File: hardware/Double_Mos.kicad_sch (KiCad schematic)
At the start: 12 parts, among them U14 AOZ5276QI, U15 AOZ5276QI

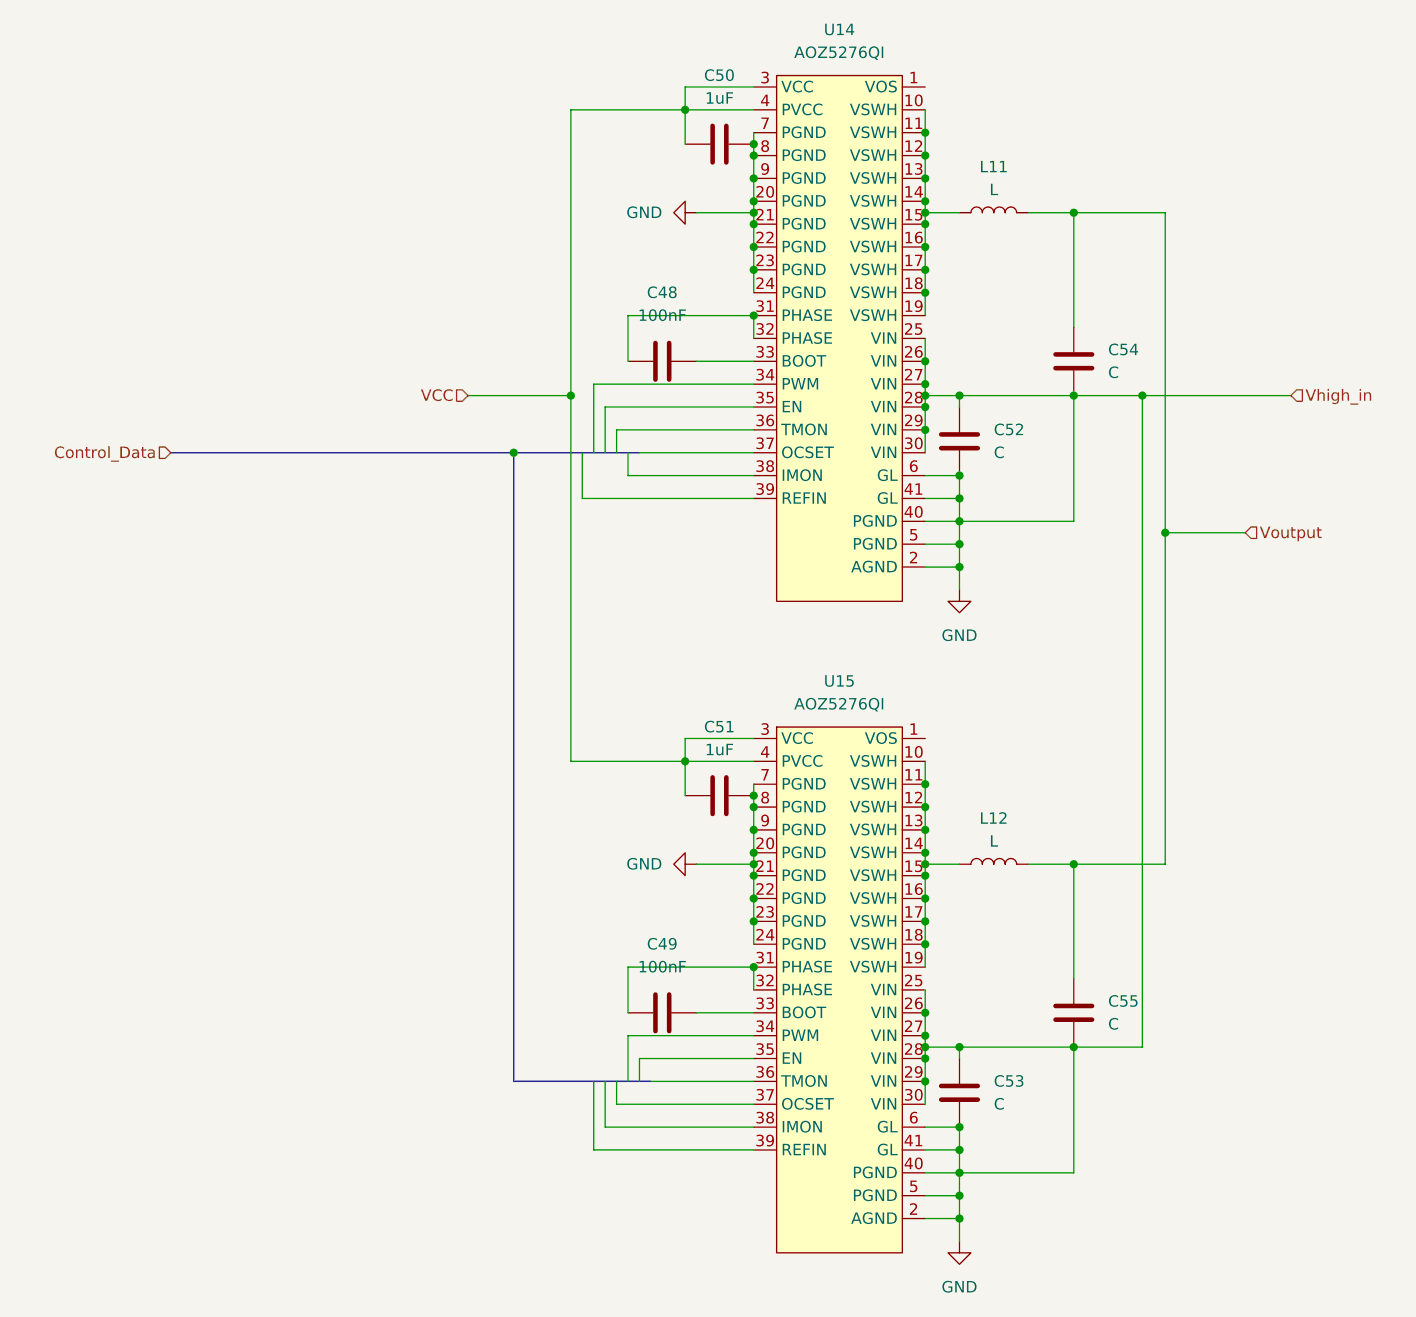
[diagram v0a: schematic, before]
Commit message: Revert "chore(schematic): Update references"
This reverts commit 2cda2d22061e90f93ddb38c43ecf32892cd7b43c.
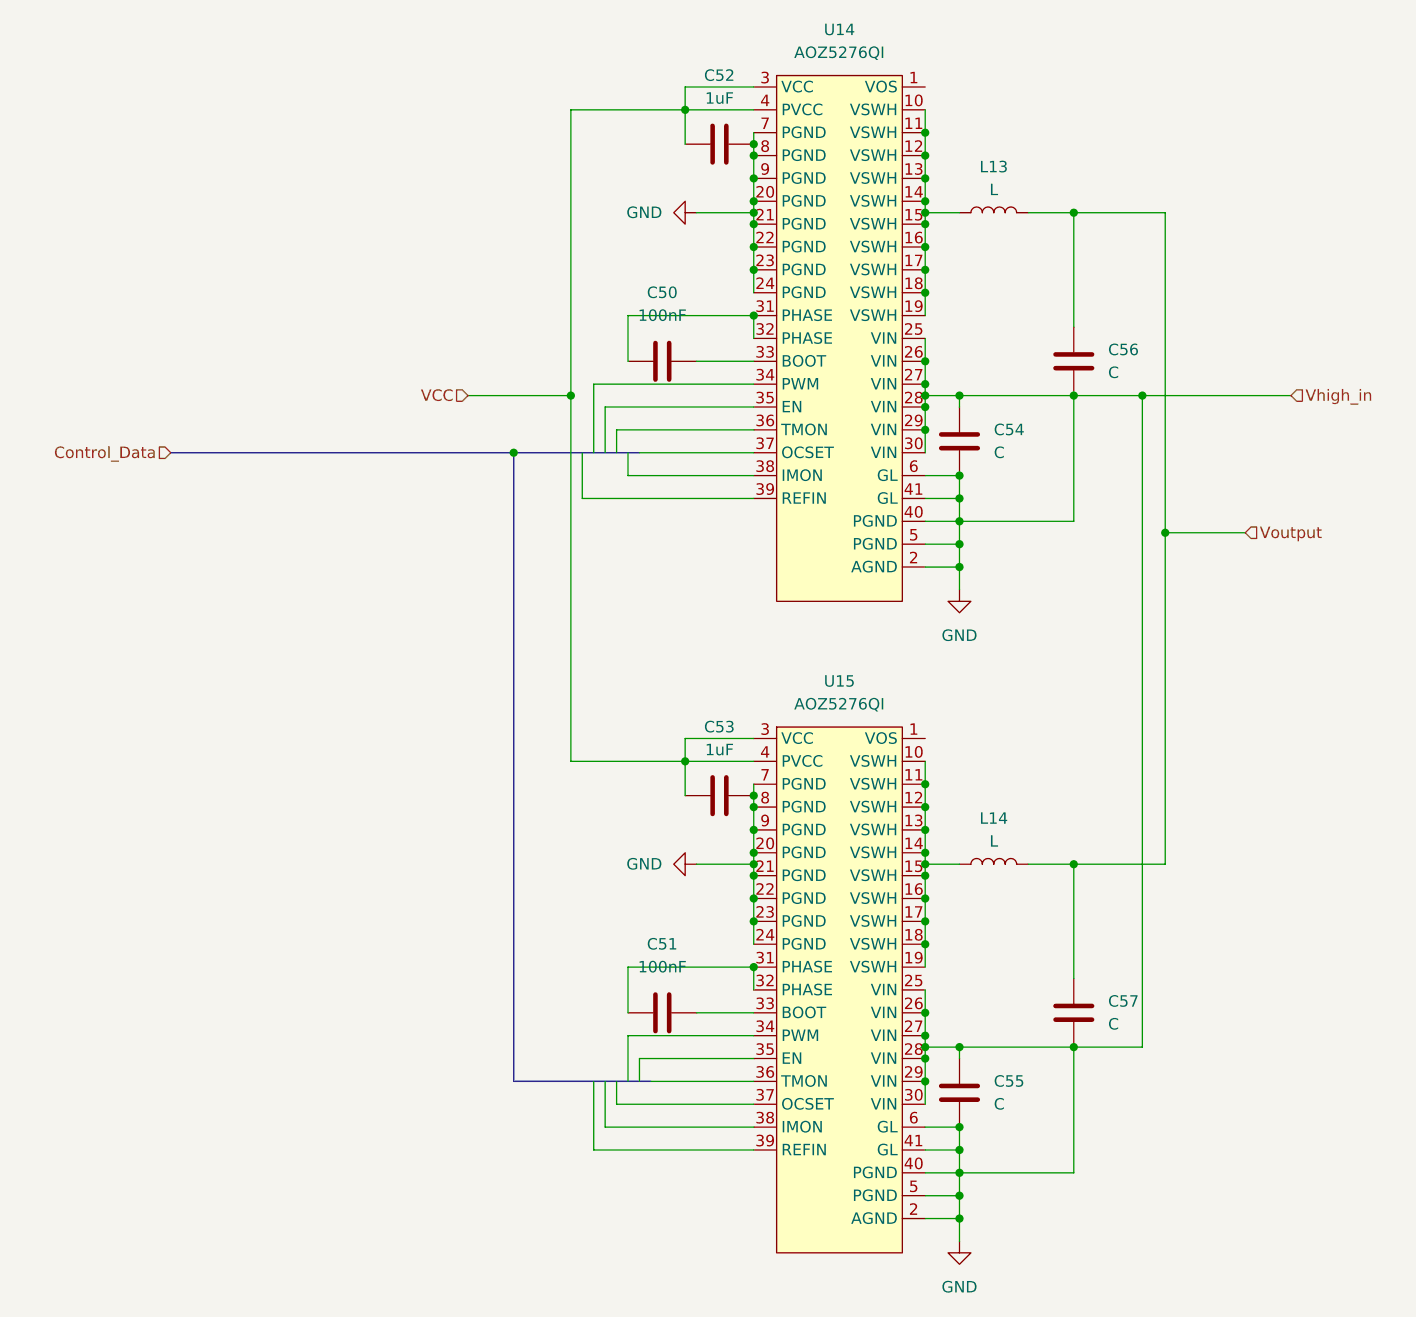
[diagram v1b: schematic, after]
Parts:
- renumbered C48 to C50, C49 to C51, C50 to C52, C51 to C53, C52 to C54, C53 to C55, C54 to C56, C55 to C57, L11 to L13, L12 to L14

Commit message: chore(schematic): Update references
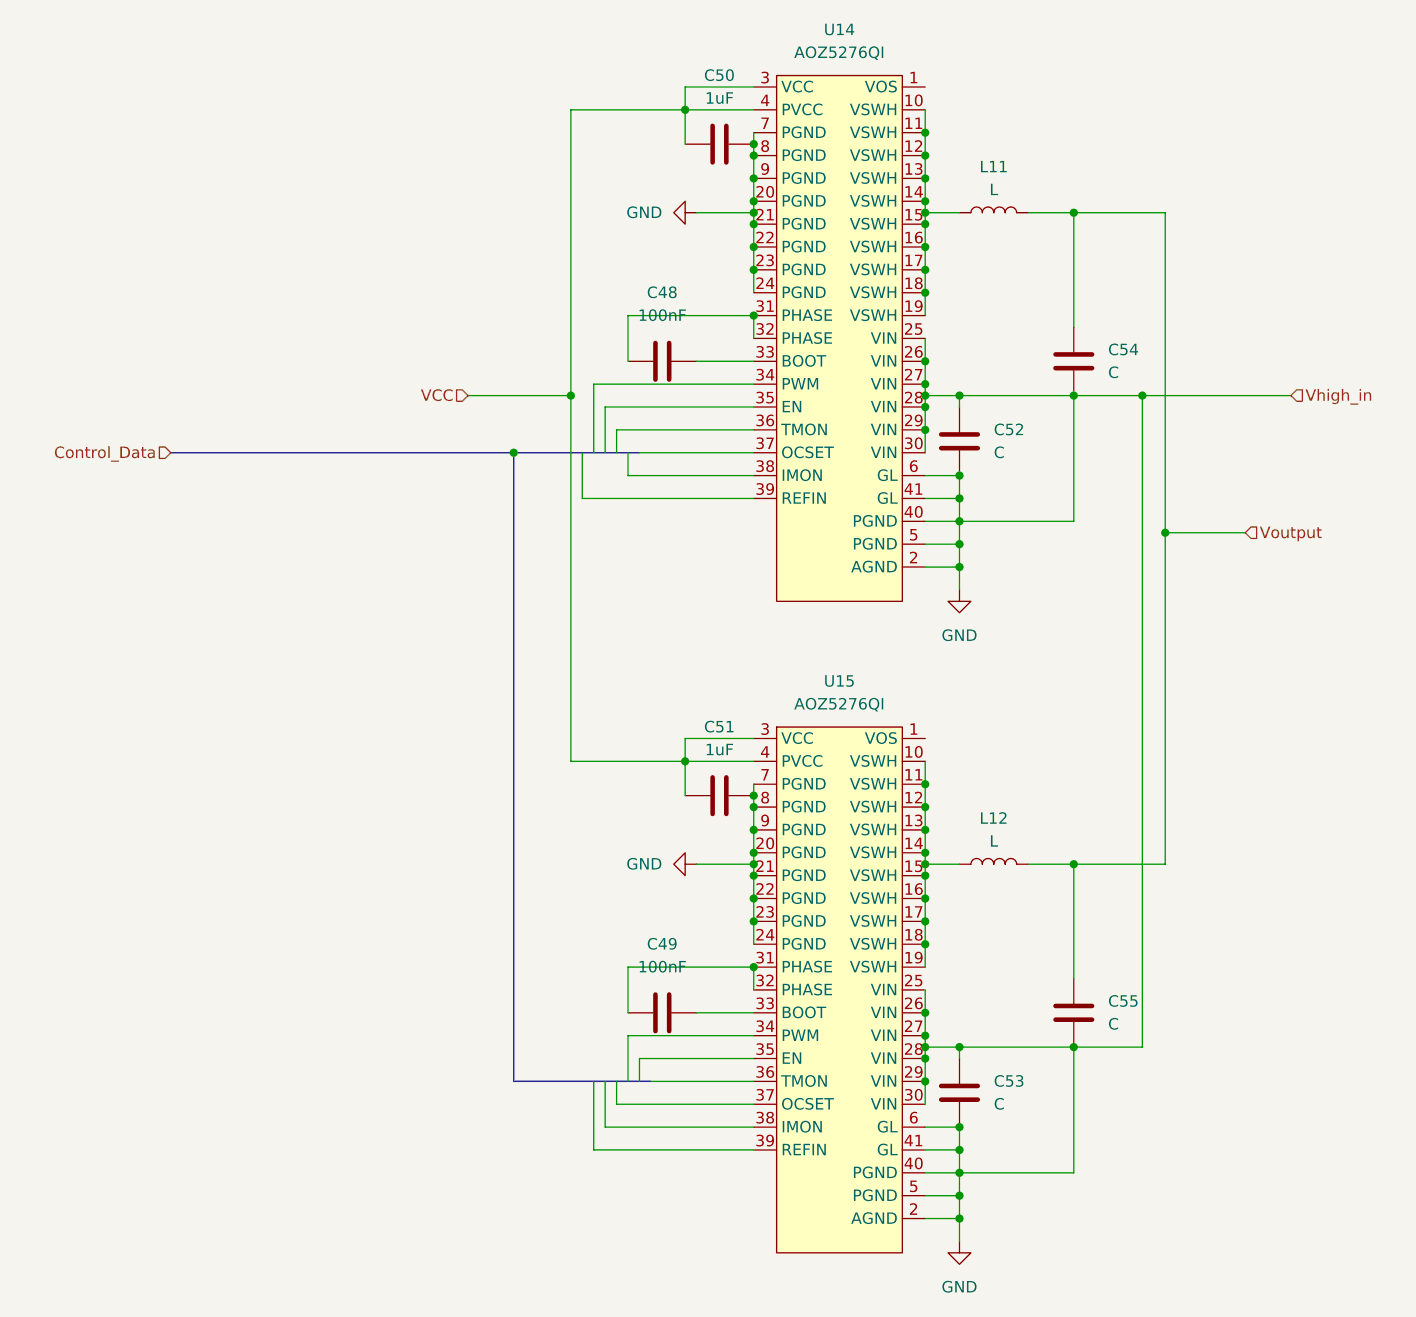
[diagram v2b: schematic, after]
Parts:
- renumbered C50 to C48, C51 to C49, C52 to C50, C53 to C51, C54 to C52, C55 to C53, C56 to C54, C57 to C55, L13 to L11, L14 to L12
